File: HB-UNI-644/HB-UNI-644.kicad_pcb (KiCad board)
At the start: 2 copper layers, 79 x 78 mm, 51 parts, among them J1 FTDI, J10 ICSP, J11 RAW, J12 Conn_Gnd, J13 Conn_NTC, J2 GS2, J3 I2C_1, J4 GS2, J5 I2C_2, J6 I2C_3, J7 I2C_4, J8 Conn_A, J9 Conn_B, Q1 IRLML6244/IRLML0030, SW1 CONFIG, U1 ATMEGA644PA-AU, U2 CC1101, U3 MAX1724, U4 LM3480-3.3, Y1 8MHz

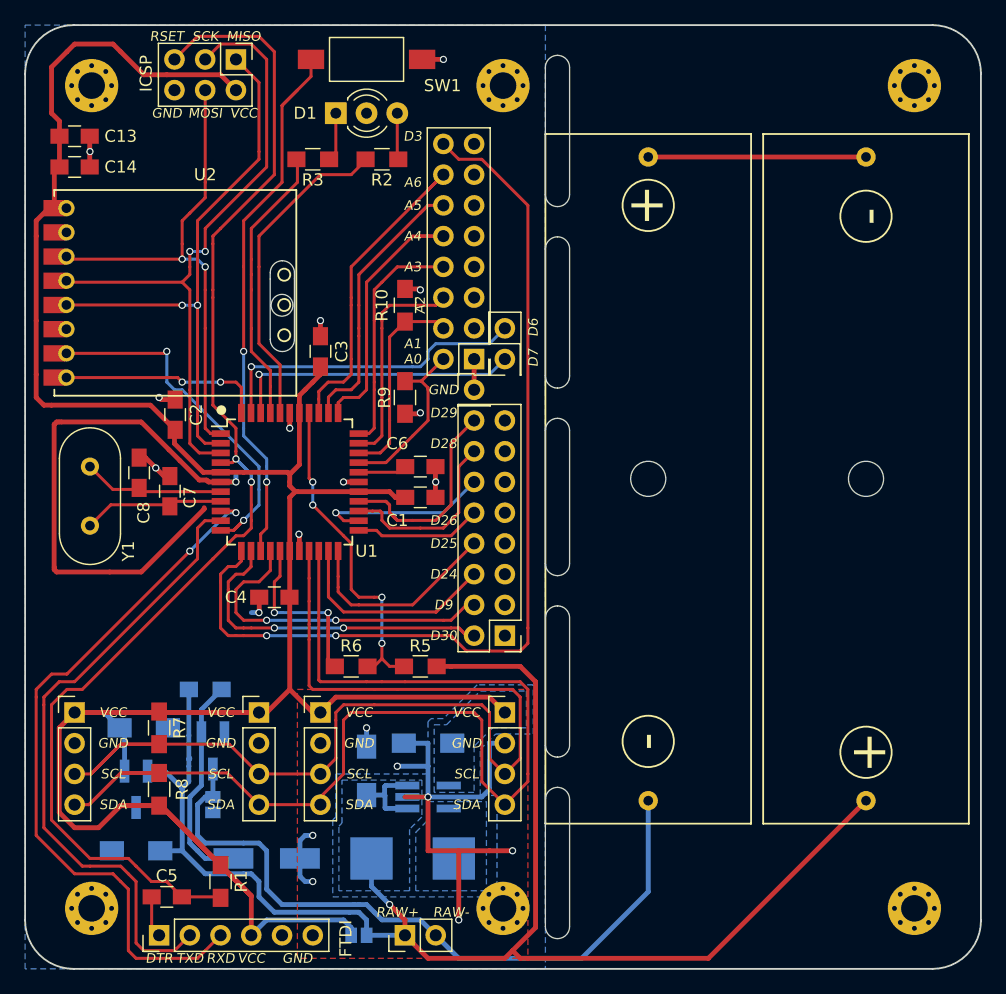
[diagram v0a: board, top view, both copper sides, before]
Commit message: Revision 2 of HB-UNI-644
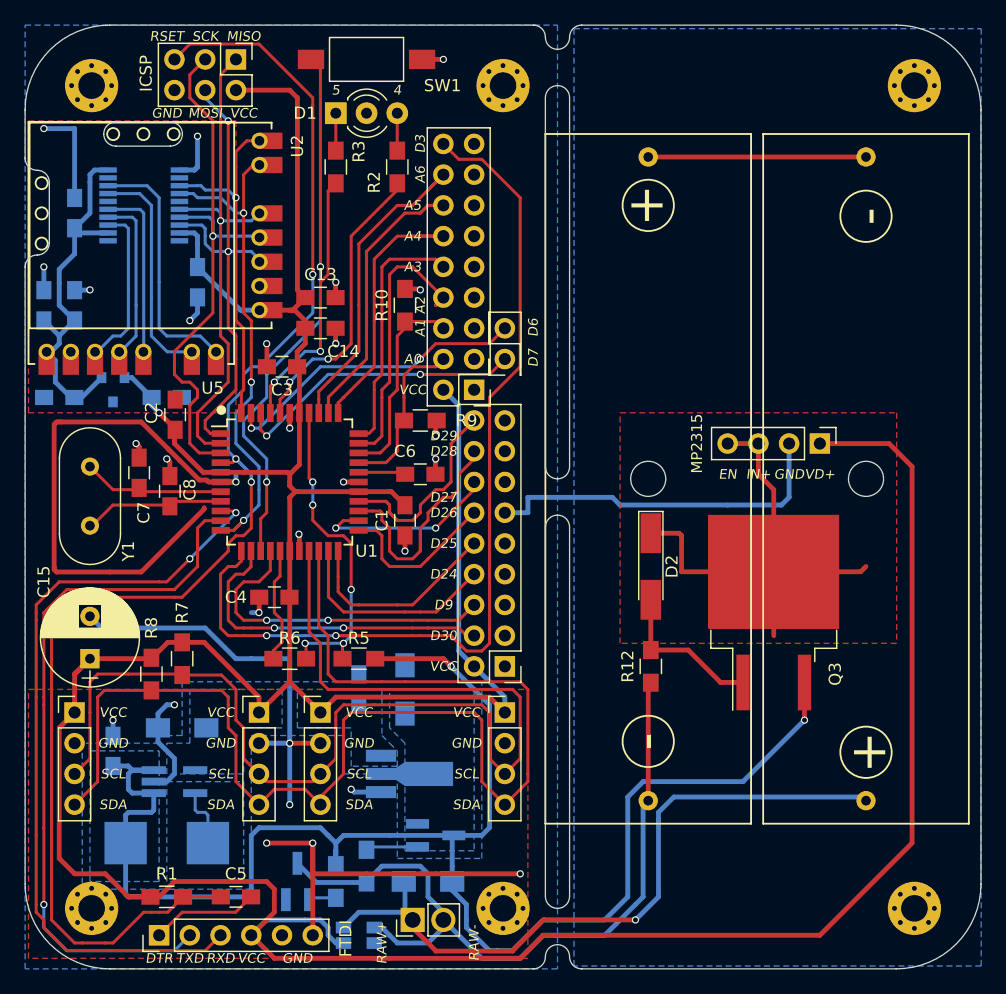
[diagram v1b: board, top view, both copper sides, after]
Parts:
- removed the REF** at (160.0, 152.0)
- removed the REF** at (102.2, 97.2)
- added C15: 1000uF, Capacitors_THT:CP_Radial_D8.0mm_P3.50mm, F.Cu at (86.4, 126.4)
- added C16: 10uF, Capacitors_SMD:C_0805_HandSoldering, B.Cu at (85.1, 97.2)
- added C17: 10nF, Capacitors_SMD:C_0805_HandSoldering, B.Cu at (82.5, 97.2)
- added C18: 10uF, Capacitors_SMD:C_0805_HandSoldering, B.Cu at (92.7, 104.8)
- added C19: 10uF, Capacitors_SMD:C_0805_HandSoldering, B.Cu at (83.8, 104.8)
- added C20: 10nF, Capacitors_SMD:C_0805_HandSoldering, B.Cu at (85.1, 89.5)
- added C21: 10nF, Capacitors_SMD:C_0805_HandSoldering, B.Cu at (95.2, 95.2)
- added F1: *, Resistors_SMD:R_1206_HandSoldering, B.Cu at (114.3, 144.8)
- added Q2: IRLML5203, TO_SOT_Packages_SMD:SOT-23_Handsoldering, B.Cu at (114.9, 141.0)
- added Q3: IRF4905S, TO_SOT_Packages_SMD:TO-263-2, F.Cu at (142.9, 122.6)
- added R11: 100K, Resistors_SMD:R_0805_HandSoldering, B.Cu at (109.2, 143.5)
- added R12: 100K, Resistors_SMD:R_0805_HandSoldering, F.Cu at (132.7, 127.0)
- added REF**: MountingHole_2.2mm_M2_Pad_Via, Mounting_Holes:MountingHole_2.2mm_M2_Pad_Via, F.Cu at (86.5, 79.0)
- added REF**: MountingHole_2.2mm_M2_Pad_Via, Mounting_Holes:MountingHole_2.2mm_M2_Pad_Via, F.Cu at (120.5, 79.0)
- added REF**: MountingHole_2.2mm_M2_Pad_Via, Mounting_Holes:MountingHole_2.2mm_M2_Pad_Via, F.Cu at (154.5, 79.0)
- added REF**: MountingHole_2.2mm_M2_Pad_Via, Mounting_Holes:MountingHole_2.2mm_M2_Pad_Via, F.Cu at (86.5, 147.0)
- added REF**: MountingHole_2.2mm_M2_Pad_Via, Mounting_Holes:MountingHole_2.2mm_M2_Pad_Via, F.Cu at (120.5, 147.0)
- added REF**: MountingHole_2.2mm_M2_Pad_Via, Mounting_Holes:MountingHole_2.2mm_M2_Pad_Via, F.Cu at (154.5, 147.0)
- added U5: CC1101, Homebrew:CC1101, F.Cu at (81.3, 103.5)
- added U6: LM3480-3.3, TO_SOT_Packages_SMD:SOT-23, B.Cu at (88.3, 104.1)
- added U7: TXS0108EPWR, Housings_SSOP:TSSOP-20_4.4x6.5mm_Pitch0.65mm, B.Cu at (90.8, 88.9)
- C12, C9: footprint Capacitors_SMD:C_1206_HandSoldering -> Capacitors_SMD:C_0805_HandSoldering
- D2: value ZMM16V -> ZMM16; moved to F.Cu
- J12: value Conn_Gnd -> Conn_01x04; footprint Pin_Headers:Pin_Header_Straight_1x01_Pitch2.54mm -> Pin_Headers:Pin_Header_Straight_1x04_Pitch2.54mm
- J8, J9: footprint Pin_Headers:Pin_Header_Straight_2x08_Pitch2.54mm -> Pin_Headers:Pin_Header_Straight_2x09_Pitch2.54mm
- Q1: value IRLML6244/IRLML0030 -> IRLML6244
- U4: value LM3480-3.3 -> HT7533-1; footprint TO_SOT_Packages_SMD:SOT-23_Handsoldering -> TO_SOT_Packages_SMD:SOT-89-3_Handsoldering
- Y1: value 8MHz -> 8MHz/16MHz
- moved D2 39.9 mm to (132.7, 118.7), turned to 270 degrees
- moved J12 28.9 mm to (146.7, 108.6), turned to 270 degrees
- moved C11 25.9 mm to (112.4, 128.9), turned to 90 degrees
- moved C14 24.3 mm to (105.4, 99.1)
- moved C13 24.3 mm to (105.4, 96.5)
- moved U2 23.9 mm to (102.9, 99.1), turned to 180 degrees
- moved U4 22.3 mm to (112.4, 135.9), turned to 0 degrees
- moved C9 21.0 mm to (88.3, 134.0)
- moved U3 21.0 mm to (93.3, 136.5)
- moved L1 20.4 mm to (92.7, 141.6)
- moved C10 20.4 mm to (94.0, 132.1)
- moved R4 19.2 mm to (106.7, 144.8), turned to 90 degrees
- moved C12 18.1 mm to (108.6, 128.9), turned to 90 degrees
- moved J2 17.2 mm to (109.9, 149.2)
- moved Q1 12.9 mm to (103.5, 144.8), turned to 90 degrees
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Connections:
- C1 pad 2: +3V3 -> VCC
- C10 pad 1: +3V3 -> VCC
- C11 pad 1: /RAW+ -> Net-(C11-Pad1)
- C12 pad 1: +3V3 -> VCC
- C13 pad 2: +3V3 -> VCC
- C14 pad 2: +3V3 -> VCC
- C2 pad 2: +3V3 -> VCC
- C3 pad 2: +3V3 -> VCC
- C4 pad 2: +3V3 -> VCC
- C9 pad 1: /RAW+ -> /RAW+FUSE
- D2 pad 2: GND -> Net-(D2-Pad2)
- J1 pad 4: +3V3 -> VCC
- J10 pad 2: +3V3 -> VCC
- J12 pad 1: GND -> VCC
- J3 pad 1: +3V3 -> VCC
- J4 pad 1: +3V3 -> VCC
- J5 pad 1: +3V3 -> VCC
- J6 pad 1: +3V3 -> VCC
- J7 pad 1: +3V3 -> VCC
- J8 pad 10: /A4 -> /A3
- J8 pad 12: /A5 -> /A4
- J8 pad 14: /A6 -> /A5
- J8 pad 16: /D3 -> /A6
- J8 pad 2: /A0 -> VCC
- J8 pad 4: /A1 -> /A0
- J8 pad 6: /A2 -> /A1
- J8 pad 8: /A3 -> /A2
- J9 pad 10: /D26 -> /D25
- J9 pad 12: /D27 -> /D26
- J9 pad 14: /D28 -> /D27
- J9 pad 16: /D29 -> /D28
- J9 pad 2: /D30 -> VCC
- J9 pad 4: /D9 -> /D30
- J9 pad 6: /D24 -> /D9
- J9 pad 8: /D25 -> /D24
- L1 pad 1: /RAW+ -> /RAW+FUSE
- Q1 pad 1: Net-(D2-Pad1) -> Net-(Q1-Pad1)
- R1 pad 1: +3V3 -> VCC
- R4 pad 1: /RAW+ -> Net-(Q1-Pad1)
- R4 pad 2: Net-(D2-Pad1) -> /RAW+FUSE
- R5 pad 2: /RAW+ -> /RAW+FUSE
- R7 pad 1: +3V3 -> VCC
- R8 pad 1: +3V3 -> VCC
- U1 pad 17: +3V3 -> VCC
- U1 pad 27: +3V3 -> VCC
- U1 pad 38: +3V3 -> VCC
- U1 pad 5: +3V3 -> VCC
- U2 pad 1: +3V3 -> VCC
- U3 pad 1: /RAW+ -> /RAW+FUSE
- U3 pad 3: /RAW+ -> /RAW+FUSE
- U3 pad 4: +3V3 -> VCC
- U4 pad 1: +3V3 -> GND
- U4 pad 2: /RAW+ -> Net-(C11-Pad1)
- U4 pad 3: GND -> VCC
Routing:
- net VCC: track 0.00 -> 320.9 mm, vias 0 -> 1
- net +3V3: track 230.4 -> 32.9 mm
- net /RAW+FUSE: track 0.00 -> 132.8 mm, vias 0 -> 2
- net GND: track 117.9 -> 195.6 mm, vias 20 -> 28
- net /RAW+: track 135.1 -> 57.5 mm
- net Net-(U5-Pad8): track 0.00 -> 21.9 mm
- net Net-(D2-Pad1): track 18.3 -> 40.0 mm
- net Net-(U5-Pad7): track 0.00 -> 19.7 mm
- net Net-(U5-Pad5): track 0.00 -> 15.6 mm
- net Net-(U5-Pad4): track 0.00 -> 14.9 mm
- net Net-(U5-Pad3): track 0.00 -> 14.6 mm
- net /RSET: track 104.8 -> 118.4 mm, vias 2 -> 3
- net /SS: track 17.9 -> 31.3 mm, vias 2 -> 1
- net Net-(D2-Pad2): track 0.00 -> 12.9 mm
- net /D2: track 30.8 -> 42.7 mm, vias 2 -> 3
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- added copper zone on B.Cu, net /RAW+FUSE
- added copper zone on B.Cu, net Net-(C11-Pad1)
- added copper zone on F.Cu, net Net-(D2-Pad1)
- added copper zone on B.Cu, net VCC
- removed copper zone on B.Cu, net +3V3
- removed copper zone on B.Cu, net /RAW+
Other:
- outline, holes or cut-outs redrawn
- board text added: "4"
- board text added: "5"
- board text added: "D27"
- board text added: "EN"
- board text added: "IN+"
- board text added: "MP2315"
- board text added: "VD+"
- board text added: "Version 2.0 - 07/2018"
- board text removed: "Version 1.0 - 06/2018"
